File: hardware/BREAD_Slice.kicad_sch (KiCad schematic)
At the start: 15 parts, among them J1 Conn_01x10_Female, J2 I2C_01x04

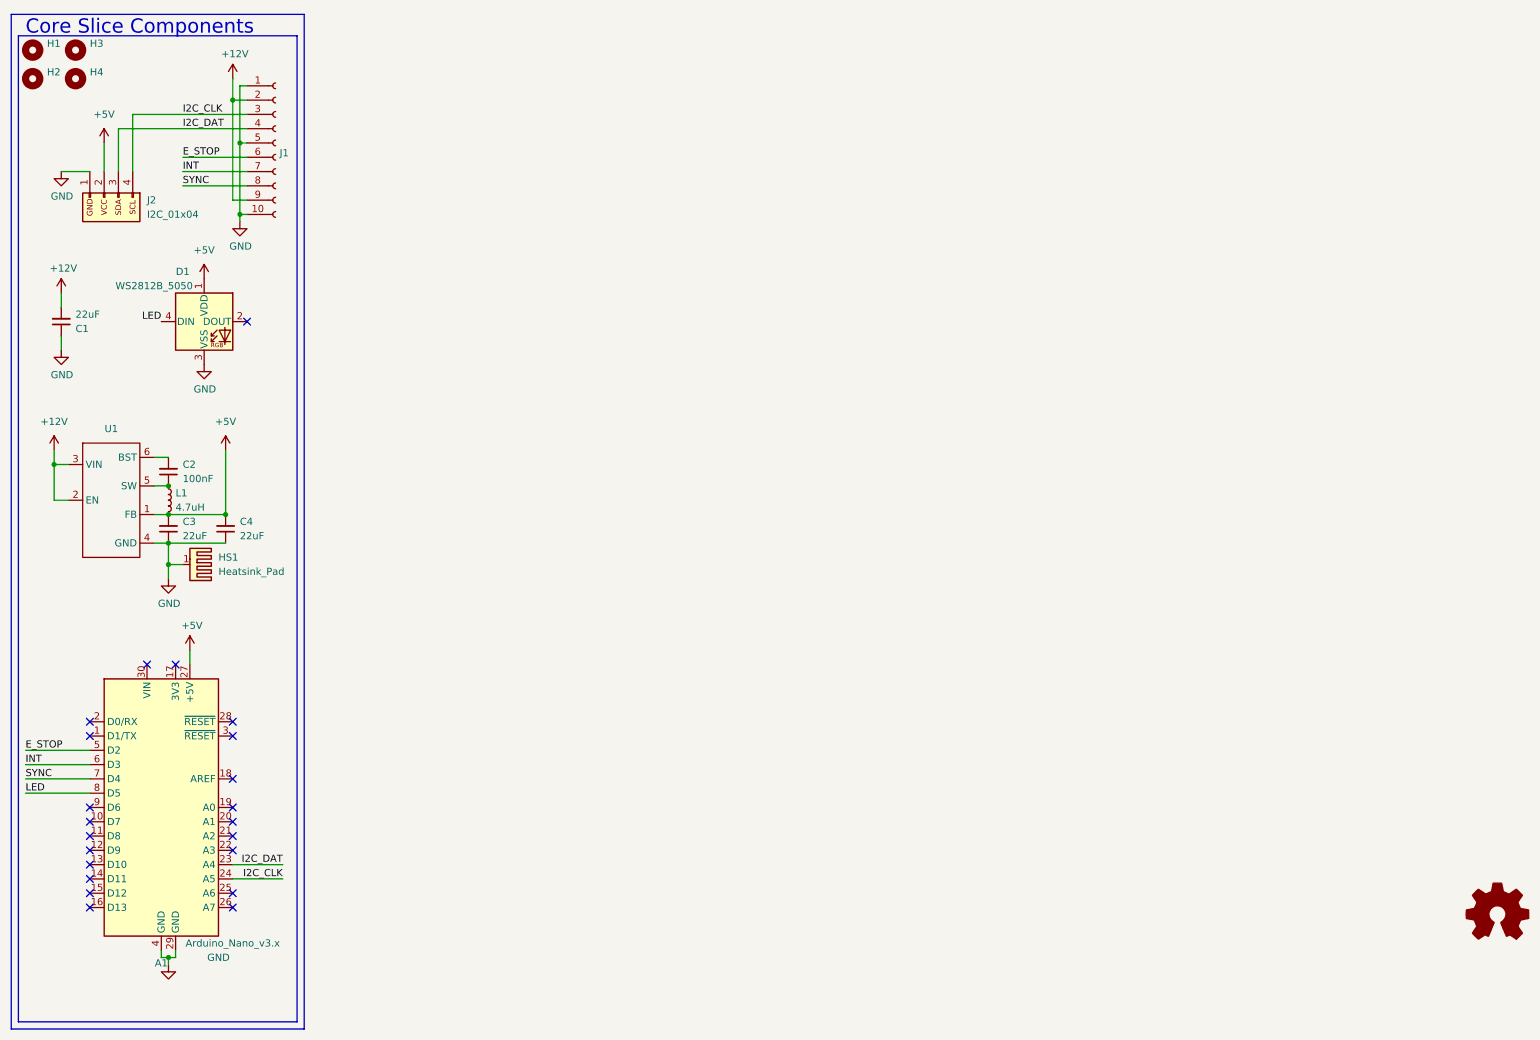
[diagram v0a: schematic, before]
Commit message: Initial commit
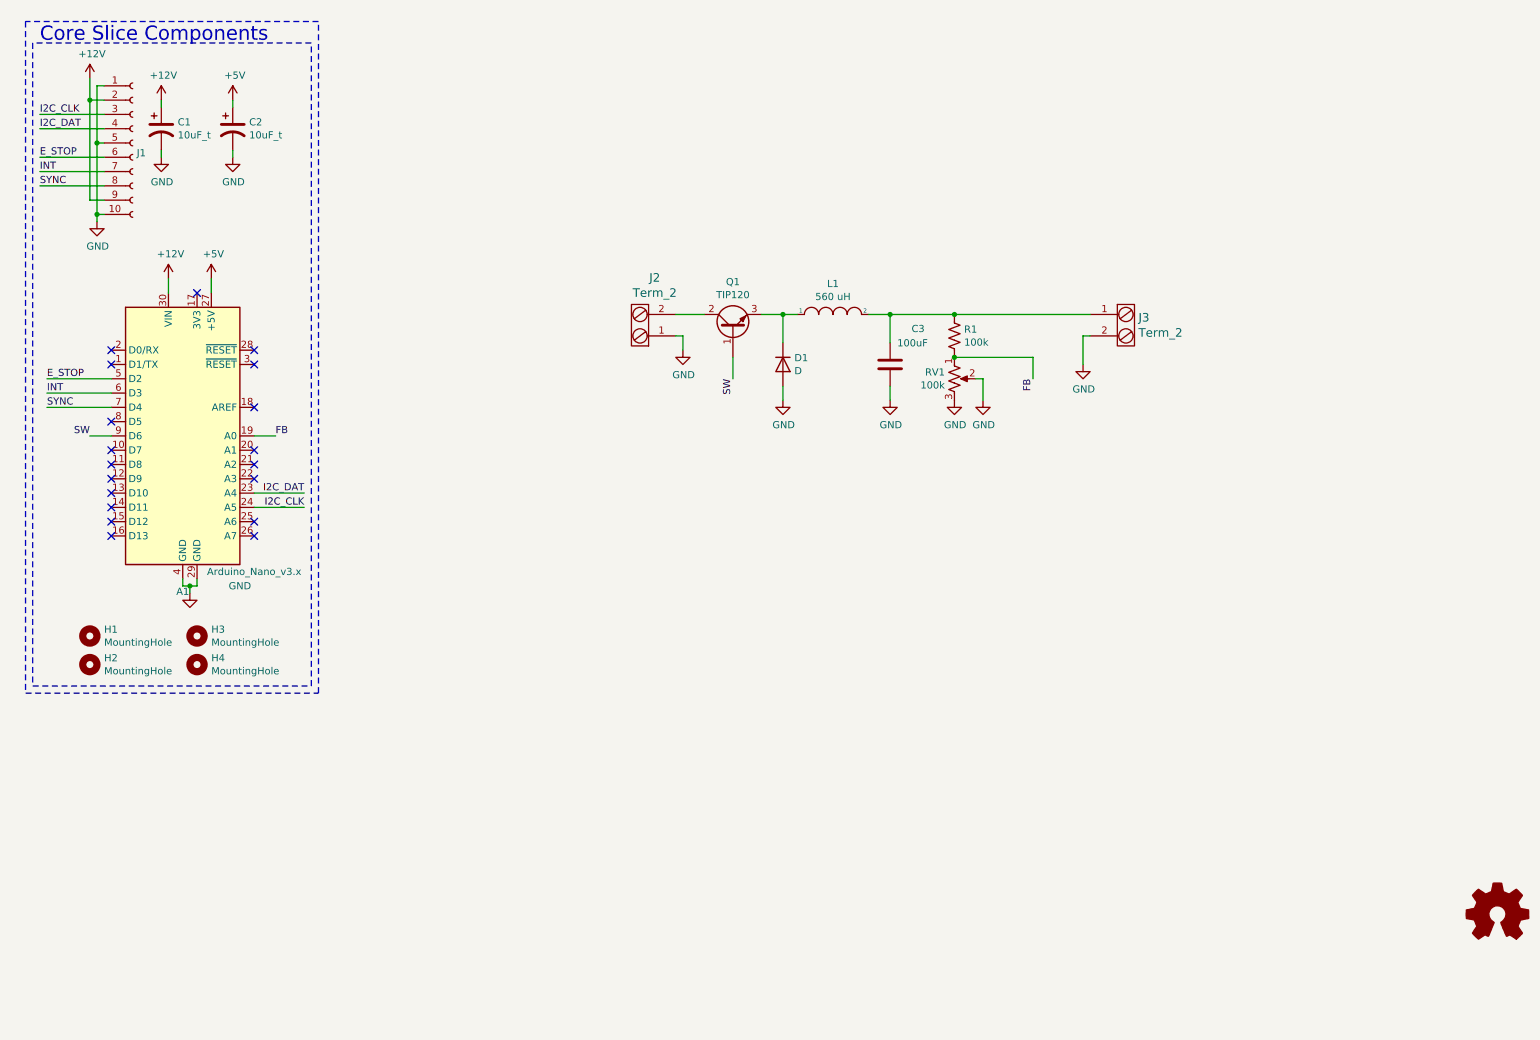
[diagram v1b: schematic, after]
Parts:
- removed C1, C3, C4: 22uF, Capacitor_SMD:C_1206_3216Metric, symbol Device:C_Small
- removed C2: 100nF, Capacitor_SMD:C_1206_3216Metric, symbol Device:C_Small
- removed D1: WS2812B_5050, SparkFun-LED:WS2812-5050-4PIN, symbol SparkFun-LED:WS2812B_5050
- removed HS1: Heatsink_Pad, SparkFun-Fuse:Thermal Pad, symbol Mechanical:Heatsink_Pad
- removed J2: I2C_01x04, Connector_JST:JST_SH_SM04B-SRSS-TB_1x04-1MP_P1.00mm_Horizontal, symbol SparkFun-Connector:I2C_01x04
- removed L1: 4.7uH, Inductor_SMD:L_1210_3225Metric, symbol Device:L_Small
- removed U1: ~, Package_TO_SOT_SMD:TSOT-23-6, symbol SparkFun-DiscreteSemi:AP63205
- added C1, C2: 10uF_t, OCI_UPL_FOOTPRINTS:C_2312, symbol BREAD_Slice-rescue:10uF_t-OCI_UPL_2_Capacitors
- added C3: 100uF, OCI_UPL_FOOTPRINTS:C_Radial_D8_L11.5_P3.5, symbol Device:C
- added D1: D, OCI_UPL_FOOTPRINTS:Diode_DO-41_SOD81_Horizontal_RM10, symbol Device:D
- added J2, J3: Term_2, OCI_UPL_FOOTPRINTS:TerminalBlock_Pheonix_MKDS1.5-2pol, symbol BREAD_Slice-rescue:Term_2-OCI_UPL_10_Connectors
- added L1: 560 uH, Inductor_THT:L_Radial_D28.0mm_P29.20mm, symbol BREAD_Slice-rescue:INDUCTOR-pspice
- added Logo1: Logo_Open_Hardware_Small, Symbol:OSHW-Symbol_6.7x6mm_SilkScreen, symbol Graphic:Logo_Open_Hardware_Small
- added Q1: TIP120, OCI_UPL_FOOTPRINTS:TO-220_Neutral123_Vertical_LargePads, symbol BREAD_Slice-rescue:TIP120-OCI_UPL_4_Semiconductors
- added R1: 100k, Resistor_THT:R_Axial_DIN0309_L9.0mm_D3.2mm_P15.24mm_Horizontal, symbol Device:R_US
- added RV1: 100k, Potentiometer_THT:Potentiometer_Bourns_3266W_Vertical, symbol BREAD_Slice-rescue:R_POT_US-Device
- H1, H4: footprint MountingHole:MountingHole_5mm -> MountingHole:MountingHole_3.2mm_M3_DIN965_Pad
- H2: renamed from H3; footprint MountingHole:MountingHole_5mm -> MountingHole:MountingHole_3.2mm_M3_DIN965_Pad
- H3: renamed from H2; footprint MountingHole:MountingHole_5mm -> MountingHole:MountingHole_3.2mm_M3_DIN965_Pad
- J1: symbol Connector:Conn_01x10_Female -> BREAD_Slice-rescue:Conn_01x10_Female-Connector
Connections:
- net +12V: now also A1.30 (VIN), C1.1
- net +5V: now also C2.1
- net GND: now also C1.2, C2.2, C3.2, D1.2 (A), J2.1, J3.2, RV1.2, RV1.3
- net FB: now reaches A1.19 (A0)
- net FB: now also R1.2, RV1.1
- net SW: now reaches A1.9 (D6)
- net SW: now also Q1.1 (B)
- net LED: no longer names the net of A1.8 (D5)
- new net: J2.2, Q1.2 (C)
- new net: D1.1 (K), L1.1, Q1.3 (E)
- new net: C3.1, J3.1, L1.2, R1.1
- no-connect marks 22 -> 19
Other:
- moved on the sheet: A1, H1, H2, H3, H4, J1
